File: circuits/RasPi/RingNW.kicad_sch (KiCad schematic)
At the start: 20 parts, among them J1 Conn_01x14_Pin, SW1 SW_SPST, U15 STM32H723VGTx, Y1 16MHz

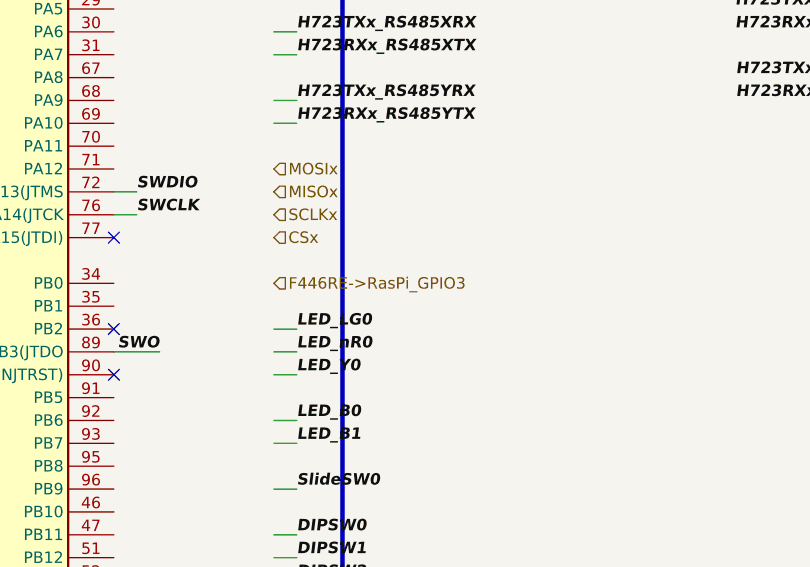
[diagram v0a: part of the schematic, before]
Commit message: raspi基板回路図
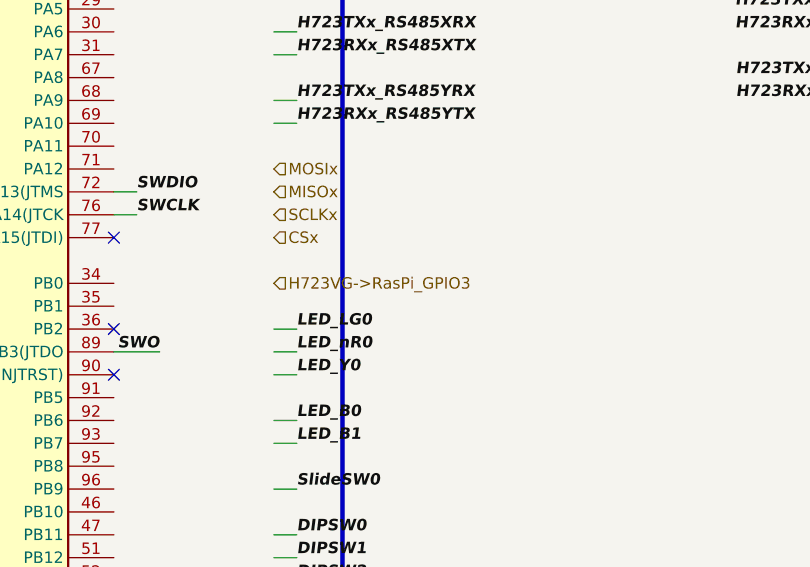
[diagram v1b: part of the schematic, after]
